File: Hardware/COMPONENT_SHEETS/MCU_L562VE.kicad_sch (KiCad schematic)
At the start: 33 parts, among them IC1 STM32L562ZET6, SW1 MCU Reset, Y3 32MHz

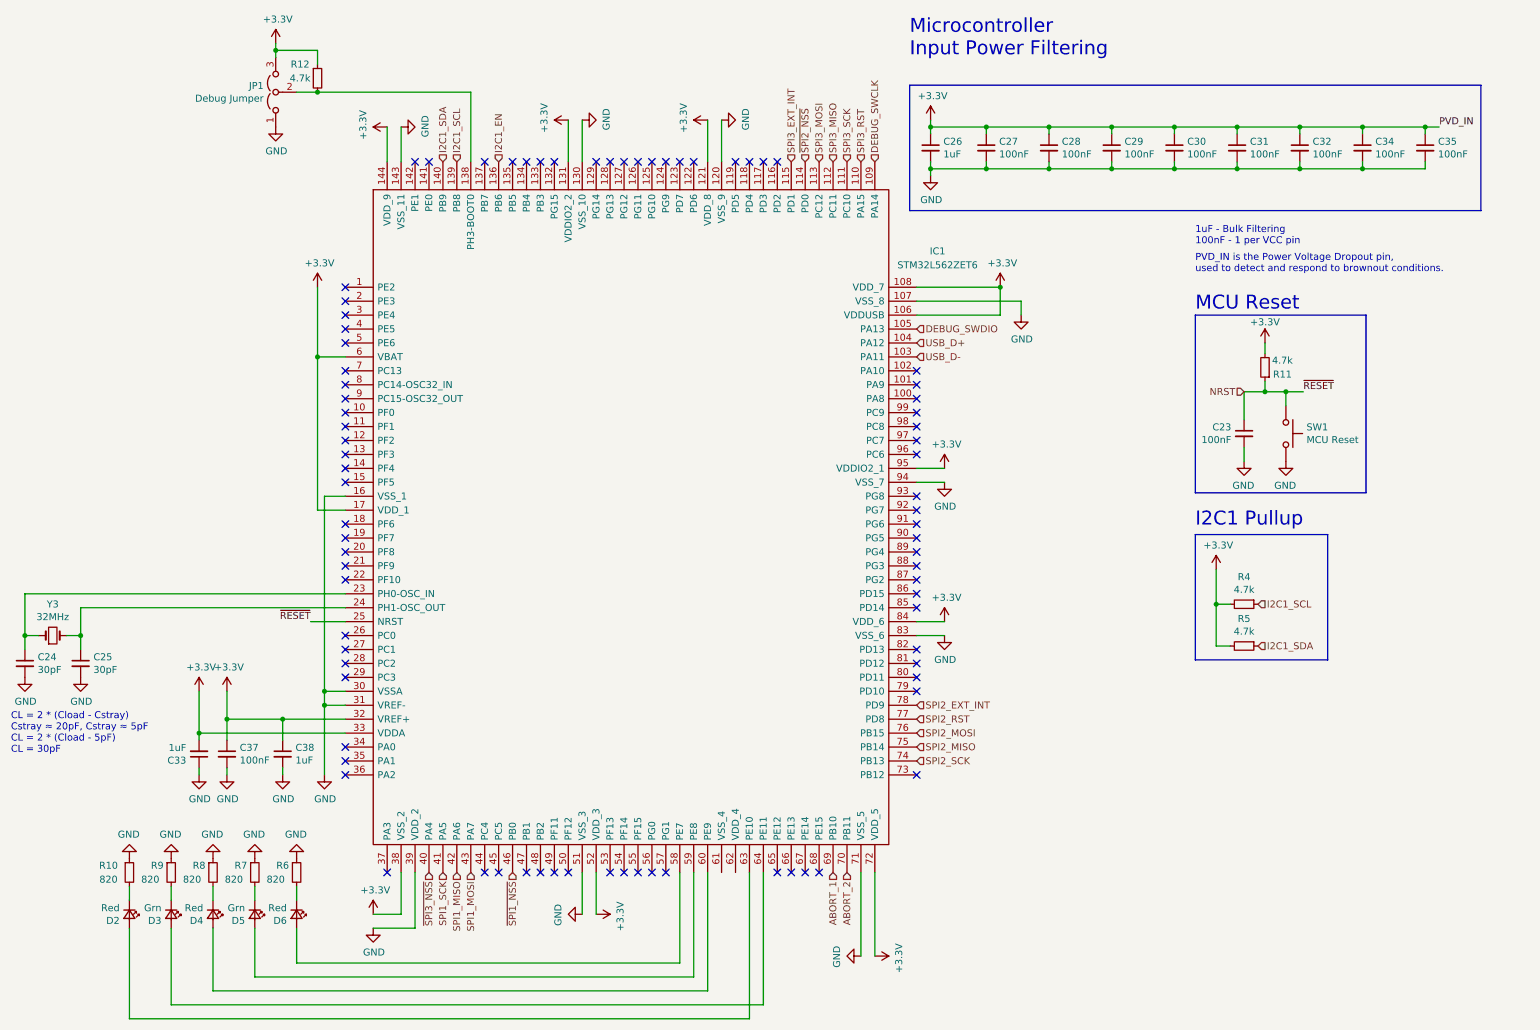
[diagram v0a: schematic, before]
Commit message: Initial routing pass
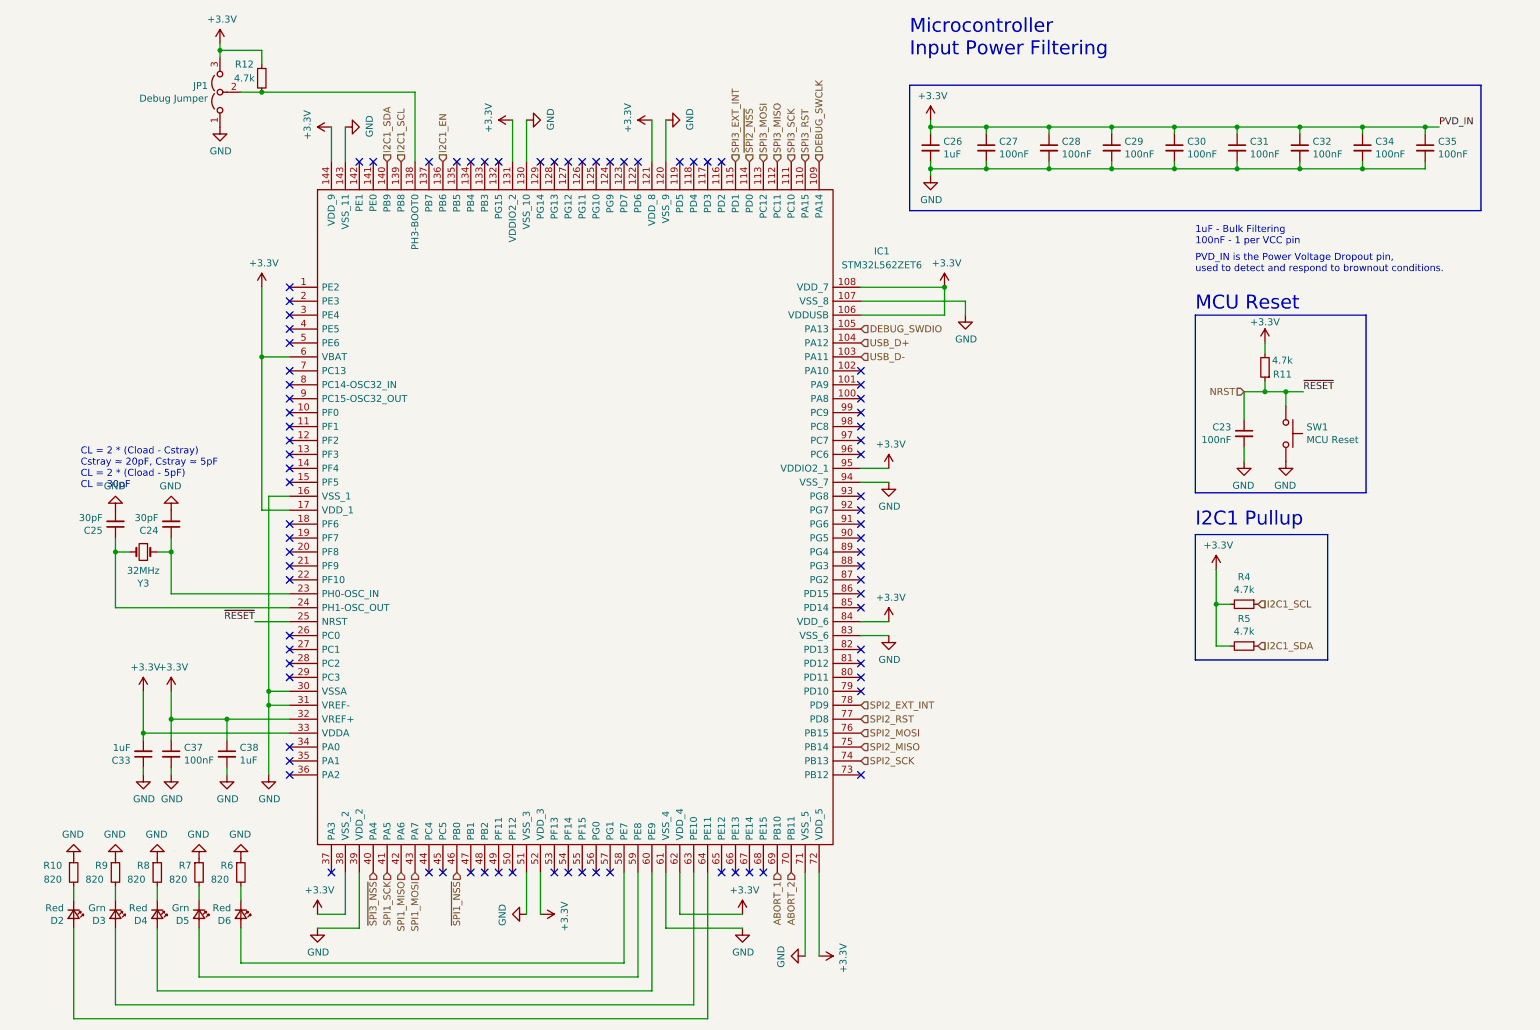
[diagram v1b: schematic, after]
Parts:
- IC1: LCSC (none) -> C1236660
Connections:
- net +3V3: now also IC1.62 (VDD_4)
- net GND: now also IC1.61 (VSS_4)
- net at D2.2 (A): now also IC1.64 (PE11); no longer IC1.63 (PE10)
- net at D3.2 (A): now also IC1.63 (PE10); no longer IC1.64 (PE11)
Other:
- moved on the sheet: C24, C25, C33, C37, C38, D2, D3, D4, D5, D6, IC1, JP1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
